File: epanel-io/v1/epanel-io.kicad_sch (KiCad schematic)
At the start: 10 parts, among them J1 Conn_01x05_Male, U1 Pico, U6 H11AA1

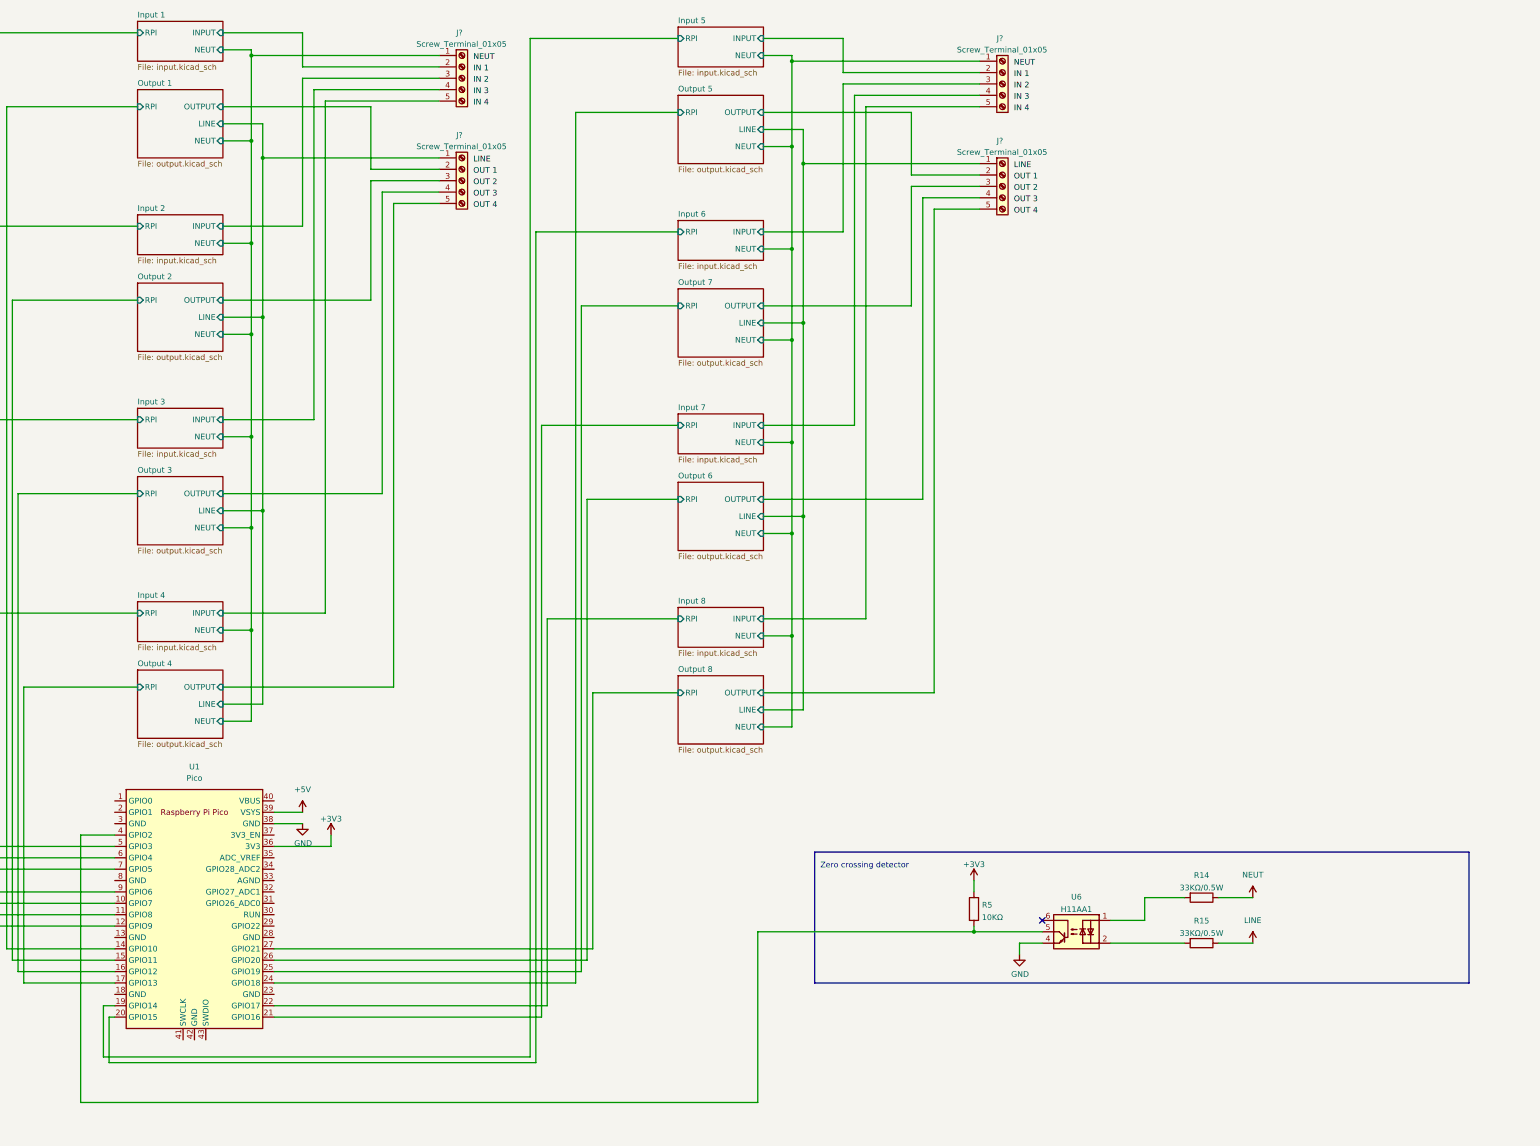
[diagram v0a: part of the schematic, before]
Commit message: wip schematic 10 io
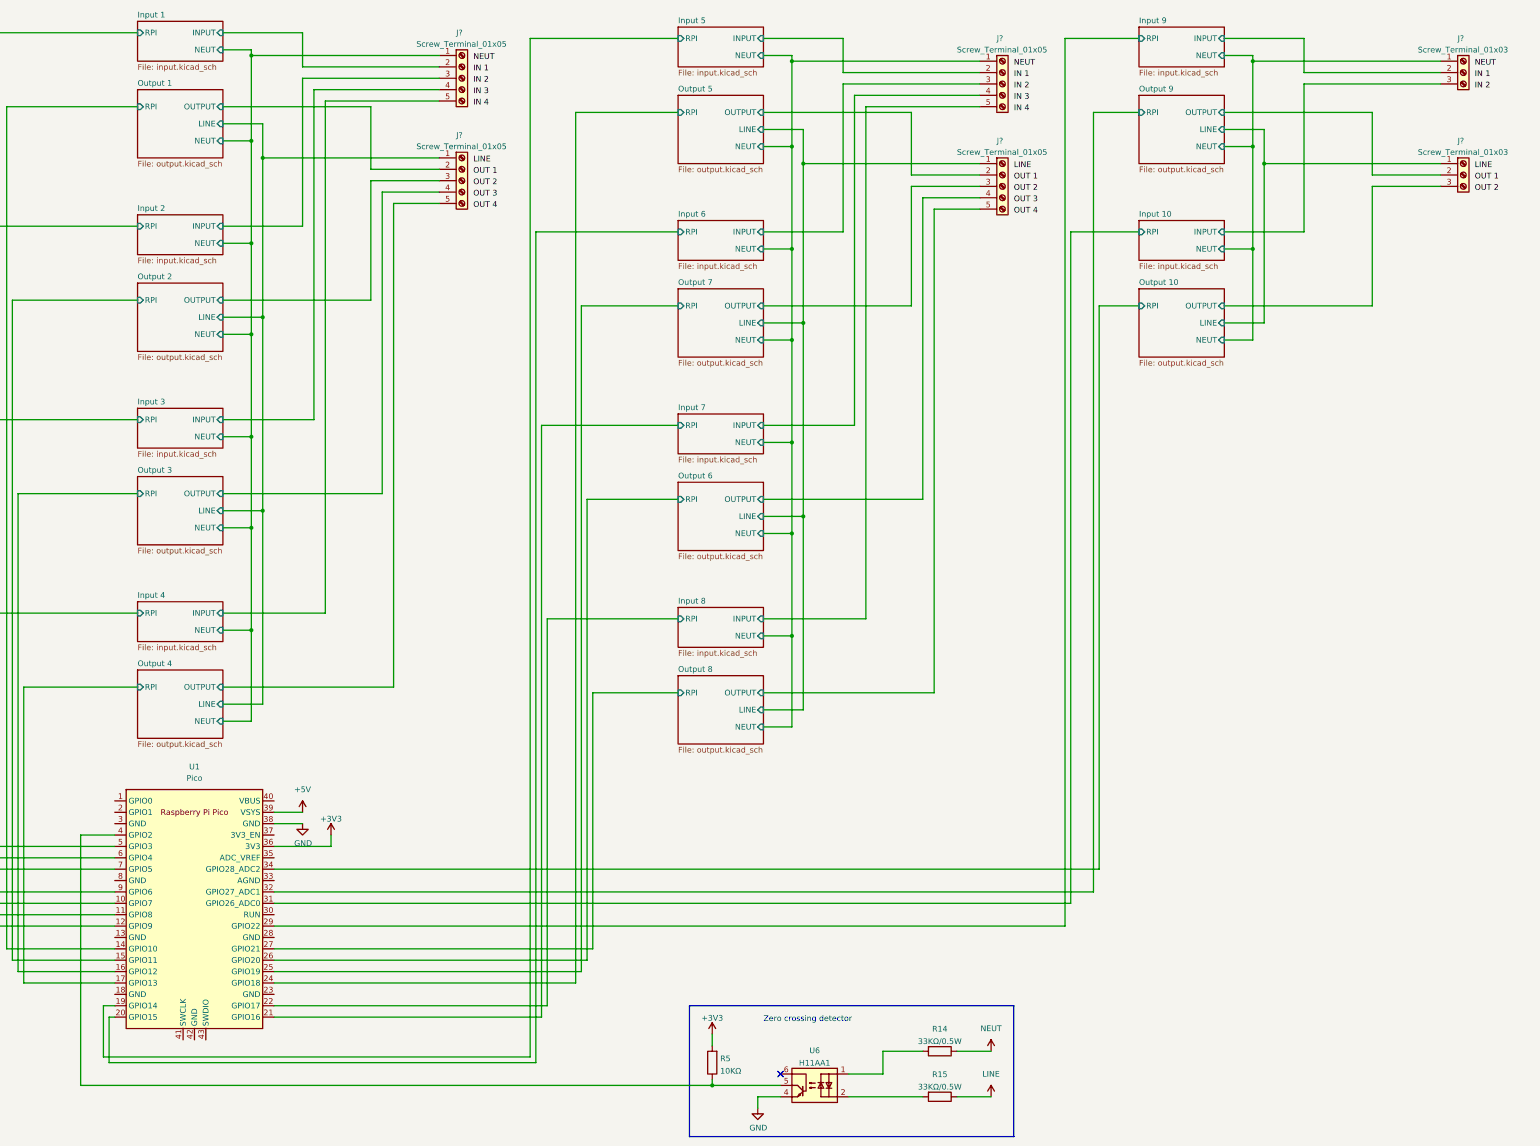
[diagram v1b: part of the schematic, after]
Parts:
- added J? (x2): Screw_Terminal_01x03, symbol Connector:Screw_Terminal_01x03
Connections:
- net Input 9/RPI: now reaches U1.29 (GPIO22)
- net Input 10/RPI: now reaches U1.31 (GPIO26_ADC0)
- net Output 9/RPI: now reaches U1.32 (GPIO27_ADC1)
- net Output 10/RPI: now reaches U1.34 (GPIO28_ADC2)
- new net Input 10/INPUT: J?.3 (Pin_3)
- new net Input 10/NEUT: J?.1 (Pin_1)
- new net Input 9/INPUT: J?.2 (Pin_2)
- new net Output 10/LINE: J?.1 (Pin_1)
- new net Output 10/OUTPUT: J?.3 (Pin_3)
- new net Output 9/OUTPUT: J?.2 (Pin_2)
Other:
- added sheet Input 10 (input.kicad_sch)
- added sheet Input 9 (input.kicad_sch)
- added sheet Output 10 (output.kicad_sch)
- added sheet Output 9 (output.kicad_sch)
- moved on the sheet: R14, R15, R5, U6
